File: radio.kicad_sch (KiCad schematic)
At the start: 28 parts, among them U301 CC1101RGPR, Y301 27MHz

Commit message: :memo: added schematic model
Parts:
- C312: LCSC C105622 -> C1671; PN CC0603JRNPO9BN470 -> CL10C470JB8NNNC
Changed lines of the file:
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@@
 			)
 		)
-		(property "LCSC" "C105622"
+		(property "LCSC" "C1671"
 			(at 246.38 109.22 0)
 			(effects
@@
 			)
 		)
-		(property "PN" "CC0603JRNPO9BN470"
+		(property "PN" "CL10C470JB8NNNC"
 			(at 246.38 109.22 0)
 			(effects

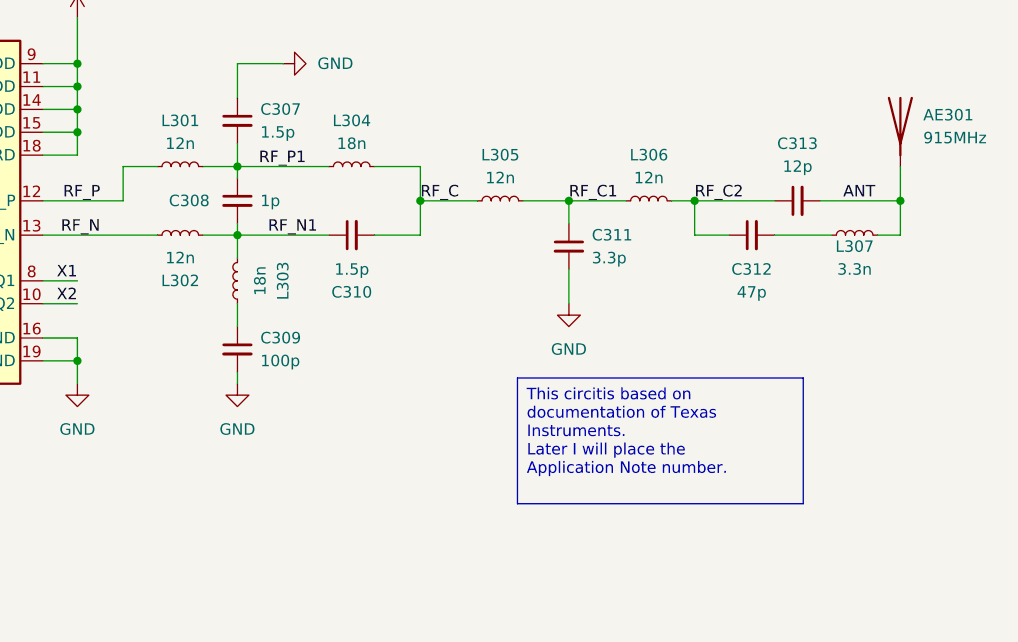
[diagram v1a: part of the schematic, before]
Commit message: small fixes
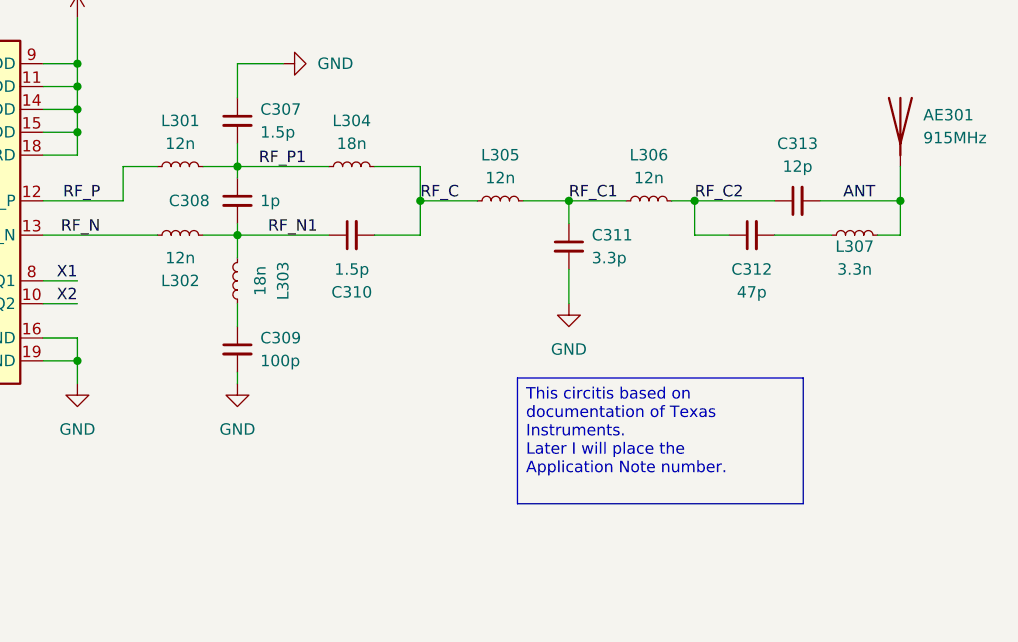
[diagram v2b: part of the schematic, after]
